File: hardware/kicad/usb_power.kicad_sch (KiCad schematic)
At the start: 15 parts, among them J1 U262-161N-4BVC11, U6 USBLC6-2P6, U7 MCP73831T-2ACI/OT

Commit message: wip
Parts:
- FB1: symbol Penguino-STM32WL-LoRa-E5-rescue:Ferrite_Bead-Device -> Device:FerriteBead
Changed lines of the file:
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@@
     )
   )
-  (symbol (lib_id "Penguino-STM32WL-LoRa-E5-rescue:Ferrite_Bead-Device") (at 87.63 30.48 90) (unit 1)
+  (symbol (lib_id "Device:FerriteBead") (at 87.63 30.48 90) (unit 1)
     (in_bom yes) (on_board yes) (dnp no)
     (property "Reference" "FB1" (at 84.455 29.21 90)
@@
       (effects (font (size 1.27 1.27)) hide)
     )
-    (property "Datasheet" "https://datasheet.lcsc.com/lcsc/2304140030_TDK-MMZ1608B601CTAH0_C97120.pdf" (at 87.63 30.48 0)
+    (property "Datasheet" "~" (at 87.63 30.48 0)
       (effects (font (size 1.27 1.27)) hide)
     )

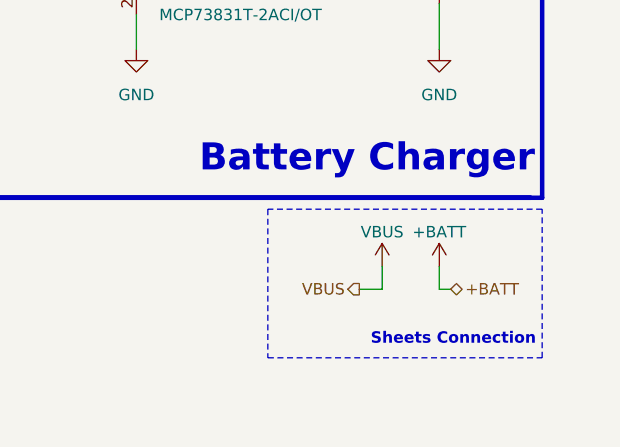
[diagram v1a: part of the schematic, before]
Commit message: revision 3 prod
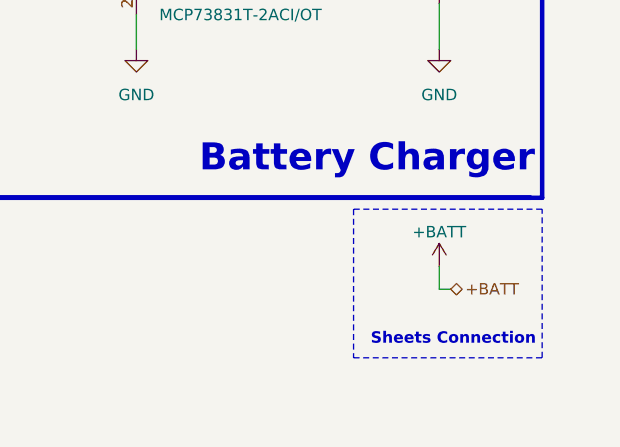
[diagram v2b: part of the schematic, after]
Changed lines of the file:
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@@
     (stroke (width 0) (type default))
   )
-  (polyline (pts (xy 165.1 69.85) (xy 165.1 86.36))
+  (polyline (pts (xy 174.625 69.85) (xy 174.625 86.36))
     (stroke (width 0) (type dash))
   )
@@
     (stroke (width 0) (type default))
   )
-  (polyline (pts (xy 195.58 69.85) (xy 165.1 69.85))
+  (polyline (pts (xy 195.58 69.85) (xy 174.625 69.85))
     (stroke (width 0) (type dash))
   )
@@
     (stroke (width 0.5) (type default))
   )
-  (wire (pts (xy 177.8 78.74) (xy 177.8 76.2))
-    (stroke (width 0) (type default))
-  )
   (polyline (pts (xy 111.125 93.98) (xy 111.125 19.05))
     (stroke (width 0.5) (type default))
@@
     (stroke (width 0) (type default))
   )
-  (wire (pts (xy 175.26 78.74) (xy 177.8 78.74))
-    (stroke (width 0) (type default))
-  )
   (wire (pts (xy 69.85 35.56) (xy 69.85 39.37))
     (stroke (width 0) (type default))
@@
     (stroke (width 0.5) (type default))
   )
-  (polyline (pts (xy 165.1 86.36) (xy 195.58 86.36))
+  (polyline (pts (xy 174.625 86.36) (xy 195.58 86.36))
     (stroke (width 0) (type dash))
   )
@@
   (hierarchical_label "+BATT" (shape bidirectional) (at 185.42 78.74 0) (fields_autoplaced)
     (effects (font (size 1.27 1.27)) (justify left))
-  )
-  (hierarchical_label "VBUS" (shape output) (at 175.26 78.74 180) (fields_autoplaced)
-    (effects (font (size 1.27 1.27)) (justify right))
   )
   (hierarchical_label "USB_D+" (shape output) (at 87.63 63.5 0) (fields_autoplaced)
@@
       (effects (font (size 1.27 1.27)) hide)
     )
-    (property "Datasheet" "~" (at 87.63 30.48 0)
+    (property "Datasheet" "https://datasheet.lcsc.com/lcsc/2304140030_TDK-MMZ1608B601CTAH0_C97120.pdf" (at 87.63 30.48 0)
       (effects (font (size 1.27 1.27)) hide)
     )
@@
         )
       )
-    )
-  )
-  (symbol (lib_id "power:VBUS") (at 177.8 76.2 0) (unit 1)
-    (in_bom yes) (on_board yes) (dnp no)
-    (property "Reference" "#PWR060" (at 177.8 80.01 0)
-      (effects (font (size 1.27 1.27)) hide)
-    )
-    (property "Value" "VBUS" (at 177.8 72.39 0)
-      (effects (font (size 1.27 1.27)))
-    )
-    (property "Footprint" "" (at 177.8 76.2 0)
-      (effects (font (size 1.27 1.27)) hide)
-    )
-    (property "Datasheet" "" (at 177.8 76.2 0)
-      (effects (font (size 1.27 1.27)) hide)
-    )
-    (pin "1")
-    (instances
-      (project "plantpal"
-        (path "/59b4123e-c7be-466b-a5db-658b8f0c1171"
-          (reference "#PWR060") (unit 1)
-        )
-        (path "/59b4123e-c7be-466b-a5db-658b8f0c1171/7fda2409-1758-4461-822b-801ba75fe202"
-          (reference "#PWR045") (unit 1)
-        )
-      )
-      (project "bwlr1e-prog"
-        (path "/630c8da6-5464-4eef-824d-89618087f4b4"
-          (reference "#PWR014") (unit 1)
-        )
-      )
-      (project "Penguino-STM32WL-LoRa-E5"
-        (path "/c338af29-f8d9-4513-836a-55ed8bfc47d3"
-          (reference "#PWR0105") (unit 1)
-        )
-      )
